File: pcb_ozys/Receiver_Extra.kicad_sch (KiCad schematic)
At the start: 16 parts, among them Q4 2N7002, Q6 AO3401A, U1 INA826AIDR

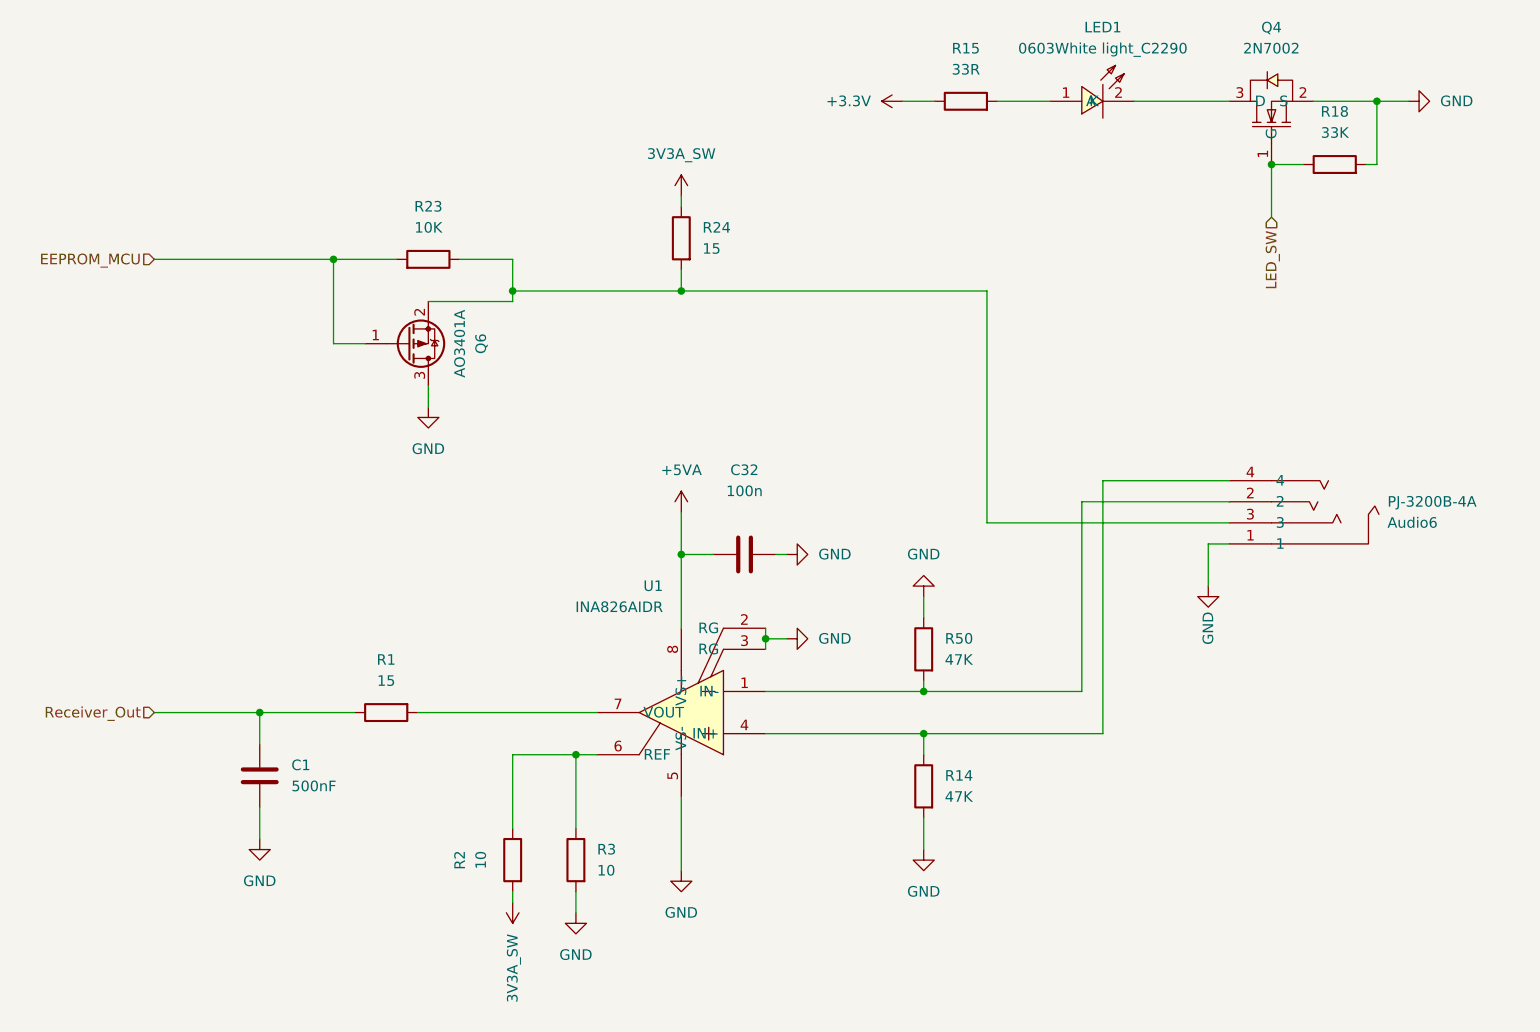
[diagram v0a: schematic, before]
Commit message: Updated Epsilon PCB and Ozys Sch
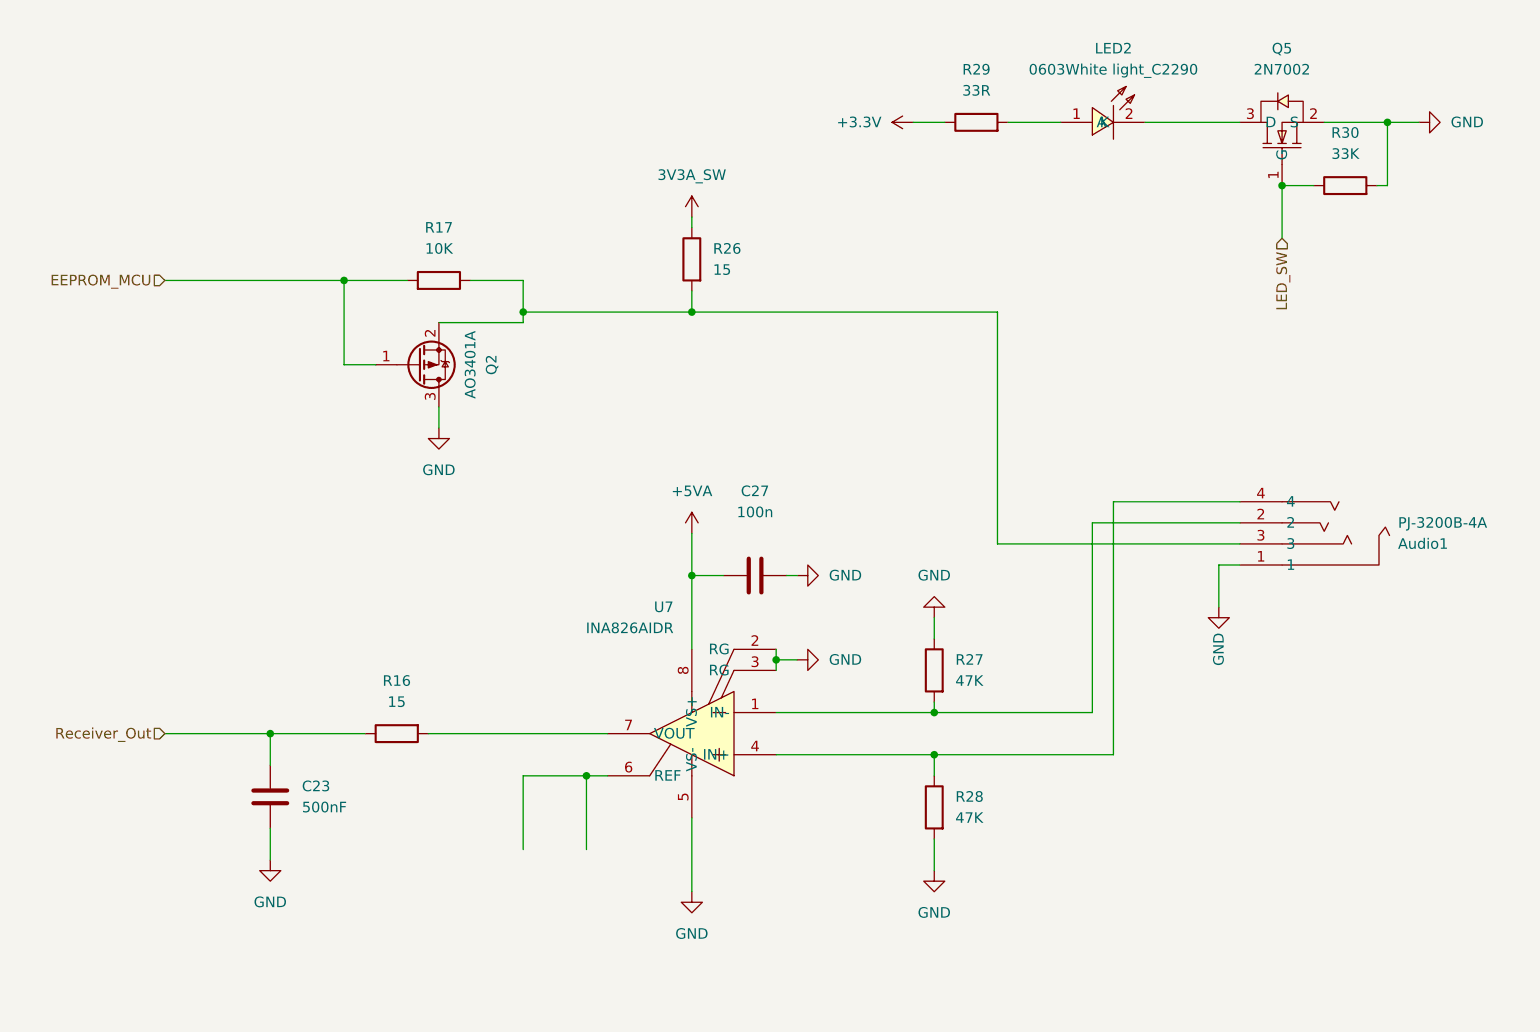
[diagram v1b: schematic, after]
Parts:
- removed Audio6: PJ-3200B-4A, Rocketry_Easyeda:AUDIO-TH_PJ-3200B-4A, symbol Rocketry_Easyeda:PJ-3200B-4A
- removed C1: 500nF, symbol Device:C
- removed C32: 100n, symbol Device:C
- removed LED1: 0603White light_C2290, Rocketry_Easyeda:LED0603-R-RD_WHITE, symbol Rocketry_Easyeda:0603Whitelight_C2290
- removed Q4: 2N7002, Rocketry_Easyeda:SOT-23-3_L2.9-W1.3-P1.90-LS2.4-BR, symbol Rocketry_Easyeda:2N7002
- removed Q6: AO3401A, Package_TO_SOT_SMD:SOT-23, symbol Transistor_FET:AO3401A
- removed R1, R24: 15, symbol Device:R
- removed R14, R50: 47K, symbol Device:R
- removed R15: 33R, Resistor_SMD:R_0402_1005Metric, symbol Device:R
- removed R18: 33K, Resistor_SMD:R_0402_1005Metric, symbol Device:R
- removed R2, R3: 10, symbol Device:R
- removed R23: 10K, symbol Device:R
- removed U1: INA826AIDR, Rocketry_Easyeda:SOIC-8_L4.9-W3.9-P1.27-LS6.0-BL, symbol Rocketry_Easyeda:INA826AIDR
- added Audio1: PJ-3200B-4A, Rocketry_Easyeda:AUDIO-TH_PJ-3200B-4A, symbol Rocketry_Easyeda:PJ-3200B-4A
- added C23: 500nF, symbol Device:C
- added C27: 100n, symbol Device:C
- added LED2: 0603White light_C2290, Rocketry_Easyeda:LED0603-R-RD_WHITE, symbol Rocketry_Easyeda:0603Whitelight_C2290
- added Q2: AO3401A, Package_TO_SOT_SMD:SOT-23, symbol Transistor_FET:AO3401A
- added Q5: 2N7002, Rocketry_Easyeda:SOT-23-3_L2.9-W1.3-P1.90-LS2.4-BR, symbol Rocketry_Easyeda:2N7002
- added R16, R26: 15, symbol Device:R
- added R17: 10K, symbol Device:R
- added R27, R28: 47K, symbol Device:R
- added R29: 33R, Resistor_SMD:R_0402_1005Metric, symbol Device:R
- added R30: 33K, Resistor_SMD:R_0402_1005Metric, symbol Device:R
- added U7: INA826AIDR, Rocketry_Easyeda:SOIC-8_L4.9-W3.9-P1.27-LS6.0-BL, symbol Rocketry_Easyeda:INA826AIDR
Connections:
- net +3.3V: now also R29.1
- net +5VA: now also C27.2, U7.8 (VS+)
- net 3V3A_SW: now also R26.1
- net EEPROM_MCU: now also Q2.1 (G), R17.2
- net GND: now also Audio1.1, C23.2, C27.1, Q2.3 (D), Q5.2 (S), R27.1, R28.2, R30.2, U7.2 (RG), U7.3 (RG), U7.5 (VS-)
- net LED_SW: now also Q5.1 (G), R30.1
- net Receiver_Out: now also C23.1, R16.1
- new net: Audio1.2, R27.2, U7.1 (IN-)
- new net: Audio1.3, Q2.2 (S), R17.1, R26.2
- new net: Audio1.4, R28.1, U7.4 (IN+)
- new net: R16.2, U7.7 (VOUT)
- new net: LED2.2 (K), Q5.3 (D)
- new net: LED2.1 (A), R29.2
